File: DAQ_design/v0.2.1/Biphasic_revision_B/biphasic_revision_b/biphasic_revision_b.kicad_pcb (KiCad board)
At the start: 2 copper layers, 64.3 x 83.6 mm, 27 parts, among them Q1 BC549, Q2 IRF9540N, Q3 IRF540N, Q4 BC549, Q5 IRF9540N, Q6 IRF540N

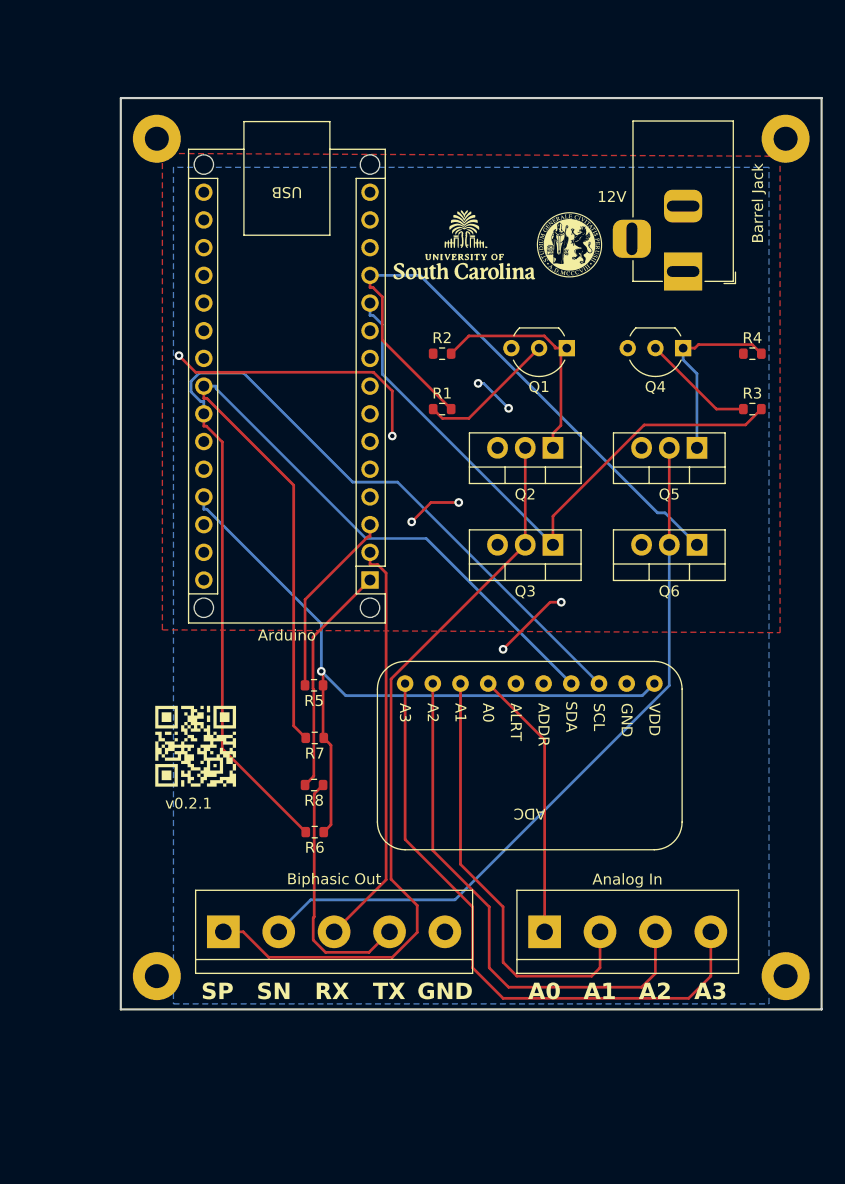
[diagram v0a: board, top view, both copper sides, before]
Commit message: naming
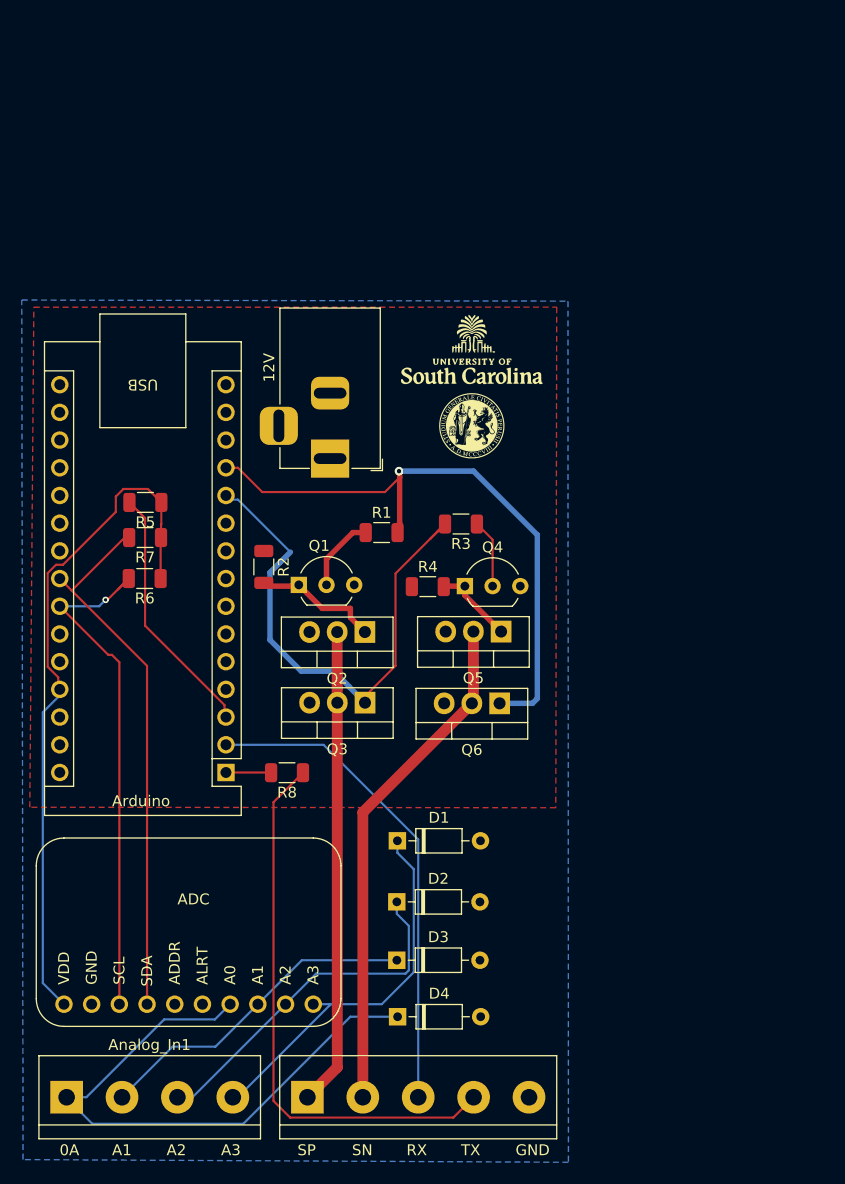
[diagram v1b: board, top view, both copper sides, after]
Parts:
- removed ADC: ADS1115IDGS, ads1115module:Adafruit_ADS1115
- removed Analog In: Screw_Terminal_01x04, TerminalBlock:TerminalBlock_bornier-4_P5.08mm
- removed Arduino: Arduino_Nano_Every, Module:Arduino_Nano_WithMountingHoles
- removed Barrel Jack: Barrel_Jack, Connector_BarrelJack:BarrelJack_Horizontal
- removed Biphasic Out: Screw_Terminal_01x05, TerminalBlock:TerminalBlock_bornier-5_P5.08mm
- removed REF1, REF2, REF3, REF4: MountingHole_2.2mm_M2_Pad, MountingHole:MountingHole_2.2mm_M2_Pad
- added A1: Arduino_Nano_Every, Module:Arduino_Nano, F.Cu at (140.4, 105.8)
- added Analog_In1: Screw_Terminal_01x04, TerminalBlock:TerminalBlock_bornier-4_P5.08mm, F.Cu at (125.8, 135.6)
- added D1: D_Zener, Diode_THT:D_DO-35_SOD27_P7.62mm_Horizontal, F.Cu at (156.2, 112.0)
- added D2: D_Zener, Diode_THT:D_DO-35_SOD27_P7.62mm_Horizontal, F.Cu at (156.1, 117.7)
- added D3: D_Zener, Diode_THT:D_DO-35_SOD27_P7.62mm_Horizontal, F.Cu at (156.1, 123.0)
- added D4: D_Zener, Diode_THT:D_DO-35_SOD27_P7.62mm_Horizontal, F.Cu at (156.2, 128.2)
- added J1: Barrel_Jack, Connector_BarrelJack:BarrelJack_Horizontal, F.Cu at (150.0, 77.0)
- added J3: Screw_Terminal_01x05, TerminalBlock:TerminalBlock_bornier-5_P5.08mm, F.Cu at (147.9, 135.6)
- added U3: ADS1115IDGS, ads1115module:Adafruit_ADS1115, F.Cu at (123.1, 129.1)
- G2: footprint boardGraphics:uofsc -> uofsc_foots:uofsc
- G3: footprint boardGraphics:upg -> uofsc_foots:upg
- G5: footprint boardGraphics:schematic -> uofsc_foots:schematic
- G7: footprint boardGraphics:github -> uofsc_foots:github; moved to B.Cu
- R1, R2, R3, R4, R5, R6, R7, R8: footprint Resistor_SMD:R_0603_1608Metric -> Resistor_SMD:R_1206_3216Metric
- moved R4 36.6 mm to (159.0, 88.7)
- moved G7 34.7 mm to (133.0, 69.0), turned to 180 degrees
- moved Q1 32.8 mm to (147.1, 88.6), turned to 0 degrees
- moved Q4 29.6 mm to (162.4, 88.7), turned to 0 degrees
- moved R3 28.7 mm to (162.0, 83.0), turned to 180 degrees
- moved R6 28.0 mm to (133.0, 88.0)
- moved R2 25.5 mm to (143.9, 86.9), turned to -90 degrees
- moved Q5 24.6 mm to (165.7, 92.9)
- moved Q2 24.1 mm to (153.2, 92.9)
- moved R7 24.1 mm to (133.0, 84.2)
- moved G5 23.4 mm to (147.0, 115.0)
- moved Q6 23.2 mm to (165.5, 99.4)
- moved R5 22.8 mm to (133.1, 81.0)
- moved Q3 22.5 mm to (153.2, 99.4)
- moved G3 18.9 mm to (163.0, 74.0)
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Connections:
- net AIN0 renamed GND
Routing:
- net GND: track 182.7 -> 0.00 mm, vias 4 -> 0
- net AIN0: track 0.00 -> 54.3 mm
- net Net-(J3-Pin_4): track 0.00 -> 51.0 mm
- net Net-(A1-SCL/A5): track 95.5 -> 48.9 mm, vias 0 -> 1
- net AIN3: track 0.00 -> 35.6 mm
- net AIN2: track 0.00 -> 32.8 mm
- net Net-(A1-SDA/A4): track 81.4 -> 49.6 mm
- net AIN1: track 0.00 -> 30.4 mm
- net VPP: track 28.8 -> 0.00 mm, vias 4 -> 0
- net SP: track 70.2 -> 45.2 mm
- net Net-(Biphasic_Out1-Pin_4): track 22.8 -> 0.00 mm
- net TX: track 21.3 -> 4.15 mm
- net SN: track 67.0 -> 50.1 mm
- net Net-(Q4-C): track 17.3 -> 7.50 mm
- net Net-(Q1-C): track 21.3 -> 11.7 mm
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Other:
- board outline removed
- board text added: "ADC"
- board text added: "Arduino"
- board text added: "H.B. Birgin David Wamai Joud Satme Austin R.J. Downey"
- board text removed: "H. B. Birgin, David Wamai, Joud Satme, Austin R. J. Downey"

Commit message: posting changes
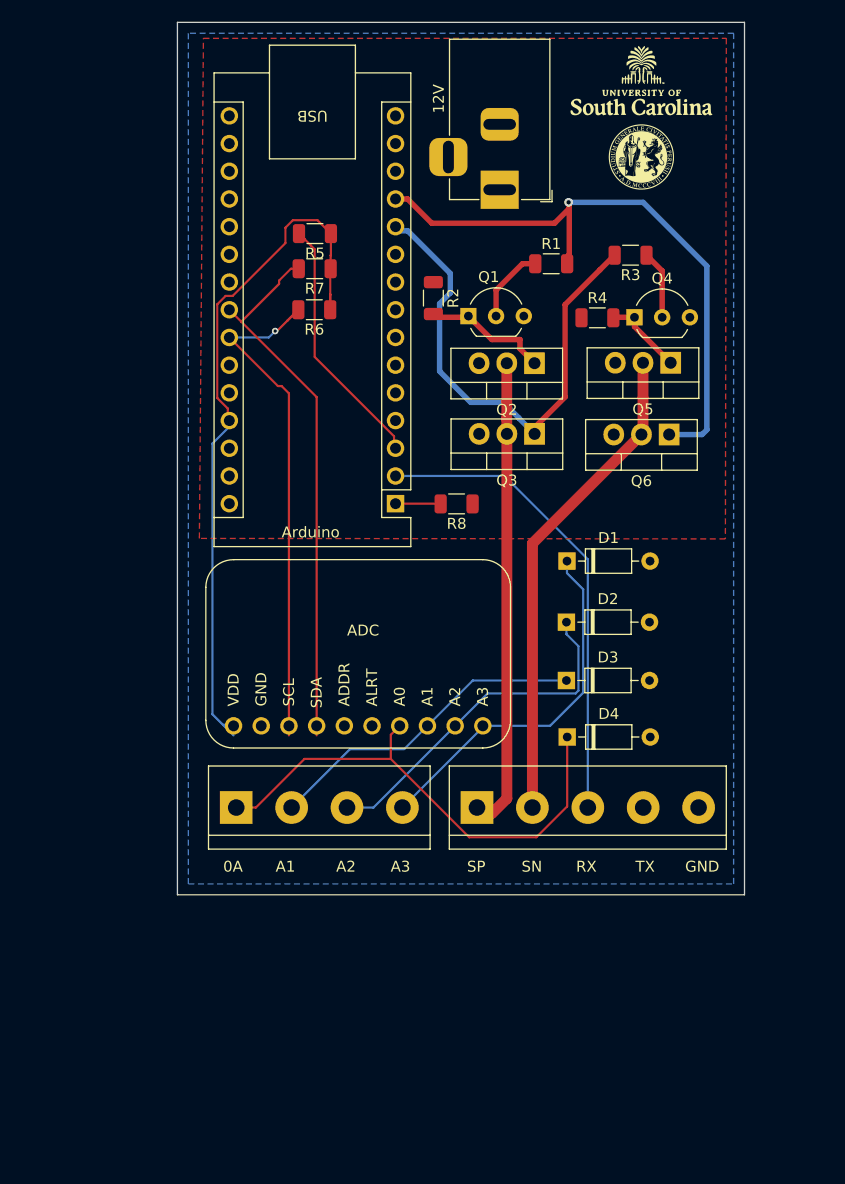
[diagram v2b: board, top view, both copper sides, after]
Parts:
- moved G7 52.8 mm to (179.0, 43.0)
- moved J3 30.8 mm to (163.5, 109.0)
- moved Analog_In1 30.8 mm to (141.4, 109.0)
- moved G5 30.2 mm to (164.0, 90.0)
- moved D4 30.0 mm to (171.7, 102.5)
- moved D1 30.0 mm to (171.7, 86.4)
- moved D2 30.0 mm to (171.7, 92.0)
- moved D3 30.0 mm to (171.7, 97.3)
- moved U3 29.9 mm to (138.6, 103.5)
- moved Q2 29.1 mm to (168.7, 68.3)
- moved Q3 29.1 mm to (168.8, 74.7)
- moved R2 29.1 mm to (159.5, 62.3)
- moved G2 29.1 mm to (178.6, 42.4)
- moved G3 29.1 mm to (178.6, 49.4)
- moved J1 29.1 mm to (165.6, 52.4)
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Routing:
- net Net-(J3-Pin_4): track 51.0 -> 0.00 mm
- net AIN0: track 54.3 -> 46.1 mm
- net VDD: track 63.4 -> 65.8 mm
- net SN: track 50.1 -> 48.2 mm
- net AIN3: track 35.6 -> 33.7 mm
- net RX: track 44.9 -> 43.6 mm
- net Net-(A1-SCL/A5): track 48.9 -> 48.1 mm
- net LOGIC2: track 50.3 -> 49.6 mm
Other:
- board outline added: 52 x 80 mm
